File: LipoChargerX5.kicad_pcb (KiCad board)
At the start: 2 copper layers, 41 parts, among them P1 Micro USB, P2 BATT_CONN, P3 BATT_CONN, P4 BATT_CONN, P5 BATT_CONN, P6 BATT_CONN, U1 MCP73831, U2 MCP73831, U3 MCP73831, U4 MCP73831, U5 MCP73831

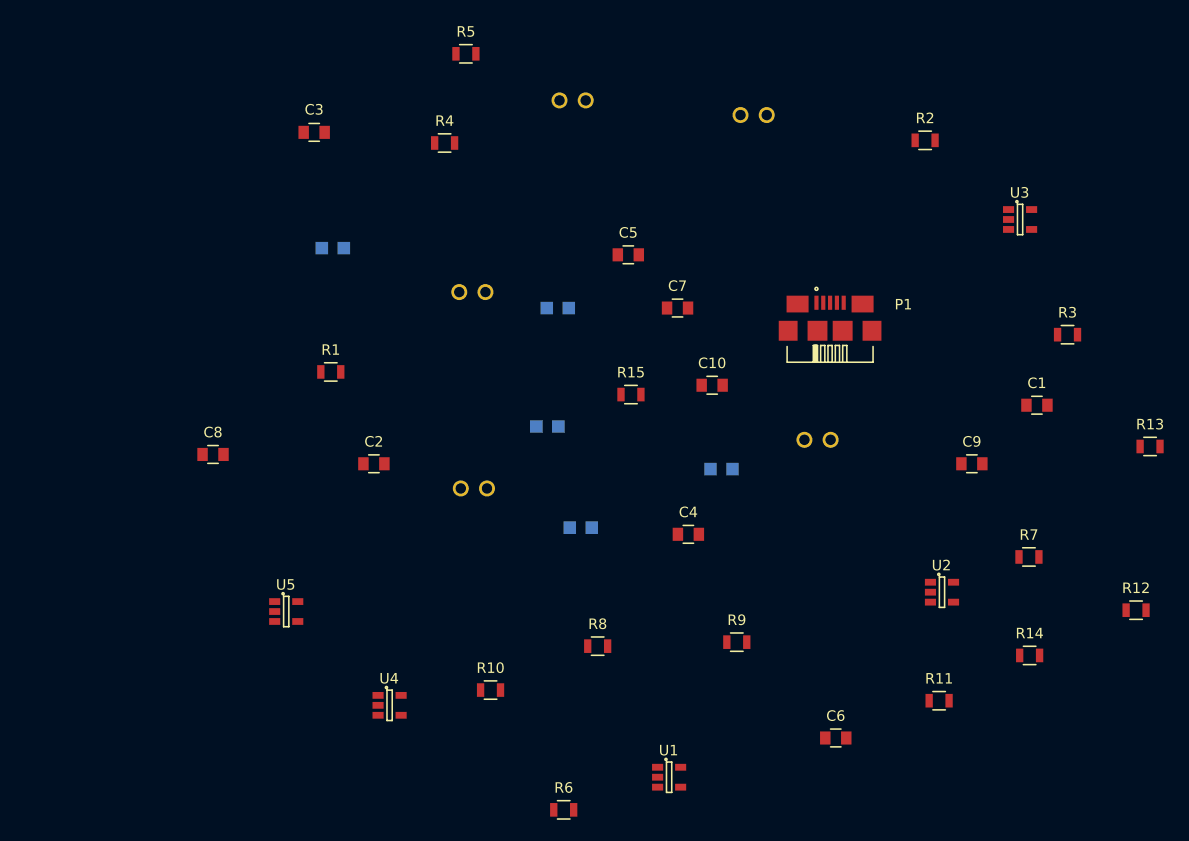
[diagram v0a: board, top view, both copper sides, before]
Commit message: Finished laying out PCB.  Generated gerbers
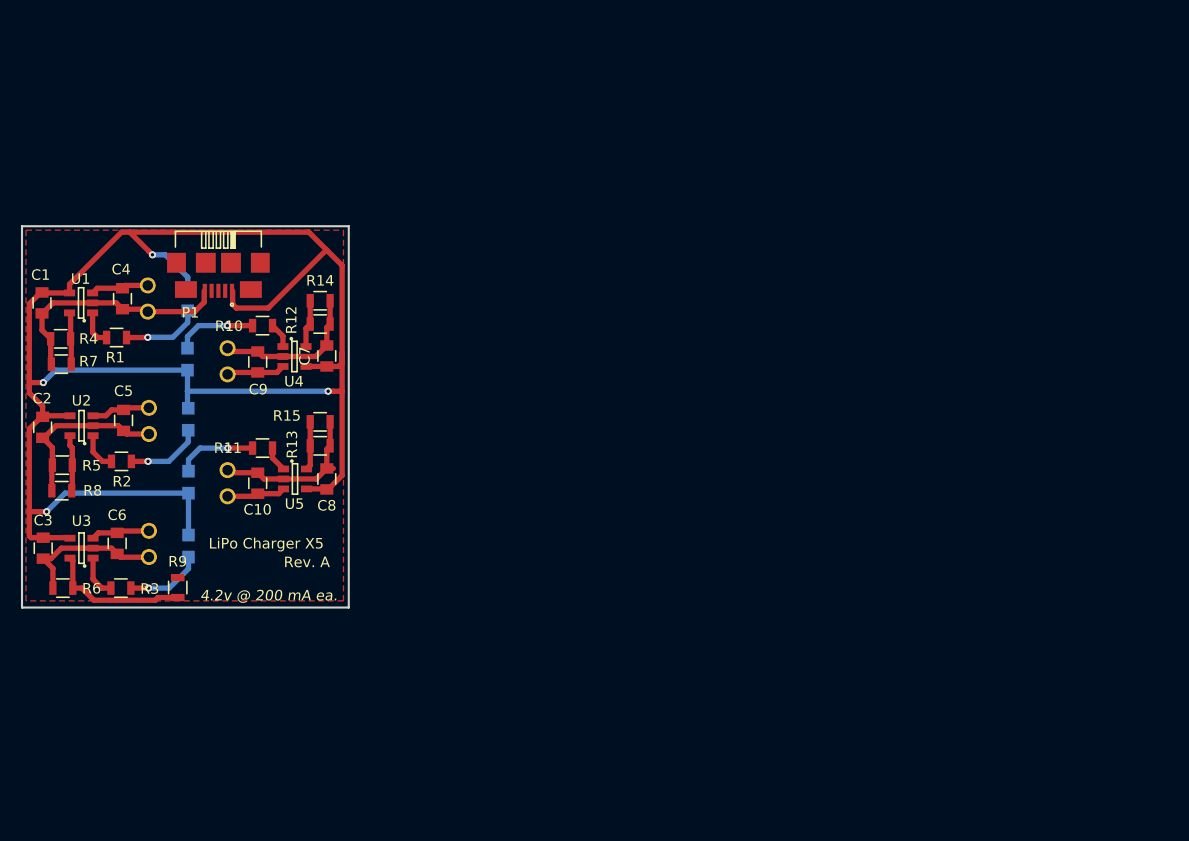
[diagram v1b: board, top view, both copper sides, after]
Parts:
- moved C1 95.4 mm to (92.7, 94.8), turned to 270 degrees
- moved U3 94.9 mm to (96.4, 118.2), turned to 180 degrees
- moved R7 94.1 mm to (94.5, 100.6), turned to 180 degrees
- moved R3 93.5 mm to (100.2, 122.0)
- moved U2 83.6 mm to (96.4, 106.5), turned to 180 degrees
- moved R2 82.6 mm to (100.2, 109.9)
- moved R12 82.5 mm to (119.2, 96.8)
- moved R13 79.2 mm to (119.2, 108.4)
- moved R14 75.7 mm to (119.2, 94.6)
- moved U1 72.1 mm to (96.4, 94.8), turned to 180 degrees
- moved C6 71.0 mm to (99.8, 117.7), turned to 270 degrees
- moved R11 68.9 mm to (113.7, 108.6), turned to 180 degrees
- moved C9 68.8 mm to (113.2, 100.4), turned to 90 degrees
- moved P4 68.3 mm to (98.6, 117.8), turned to 270 degrees
- moved P3 66.8 mm to (98.6, 106.0), turned to 270 degrees
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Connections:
- P1 pad : (no net) -> GND
- P1 pad 4: GND -> (no net)
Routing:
- net +5V: track 0.00 -> 168.2 mm, vias 0 -> 4
- net GND: track 0.00 -> 82.6 mm
- net Net-(R6-Pad1): track 0.00 -> 13.6 mm
- net Net-(D4-Pad1): track 0.00 -> 7.75 mm, vias 0 -> 1
- net Net-(D5-Pad1): track 0.00 -> 7.67 mm, vias 0 -> 1
- net Net-(D1-Pad1): track 0.00 -> 7.54 mm, vias 0 -> 1
- net Net-(D3-Pad1): track 0.00 -> 7.38 mm, vias 0 -> 1
- net Net-(D2-Pad1): track 0.00 -> 7.30 mm, vias 0 -> 1
- net Net-(C5-Pad1): track 0.00 -> 5.65 mm
- net Net-(C10-Pad1): track 0.00 -> 5.63 mm
- net Net-(C9-Pad1): track 0.00 -> 5.60 mm
- net Net-(C4-Pad1): track 0.00 -> 5.56 mm
- net Net-(R5-Pad1): track 0.00 -> 5.37 mm
- net Net-(C6-Pad1): track 0.00 -> 5.33 mm
- net Net-(R4-Pad1): track 0.00 -> 4.96 mm
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- added copper zone on F.Cu, net GND
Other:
- board outline added: 31.2 x 36.4 mm
- net class Default: clearance 0.2 -> 0.1524; trace_width 0.25 -> 0.1524; via_dia 0.6 -> 0.6858; via_drill 0.4 -> 0.3302
- rule trace_clearance: 0.2 -> 0.1524
- rule trace_min: 0.2 -> 0.1524
- rule via_min_drill: 0.3 -> 0.3302
- rule via_min_size: 0.4 -> 0.6858
- board text added: "4.2v @ 200 mA ea."
- board text added: "LiPo Charger X5"
- board text added: "Rev. A"
